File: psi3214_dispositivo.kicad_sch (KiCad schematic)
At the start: 29 parts, among them J1 Screw_Terminal_01x02, J2 Screw_Terminal_01x03, J3 Conn_01x02_Socket, J4 Conn_01x03, J5 Conn_01x02_Socket, J6 Screw_Terminal_01x02, U1 TL072_sim

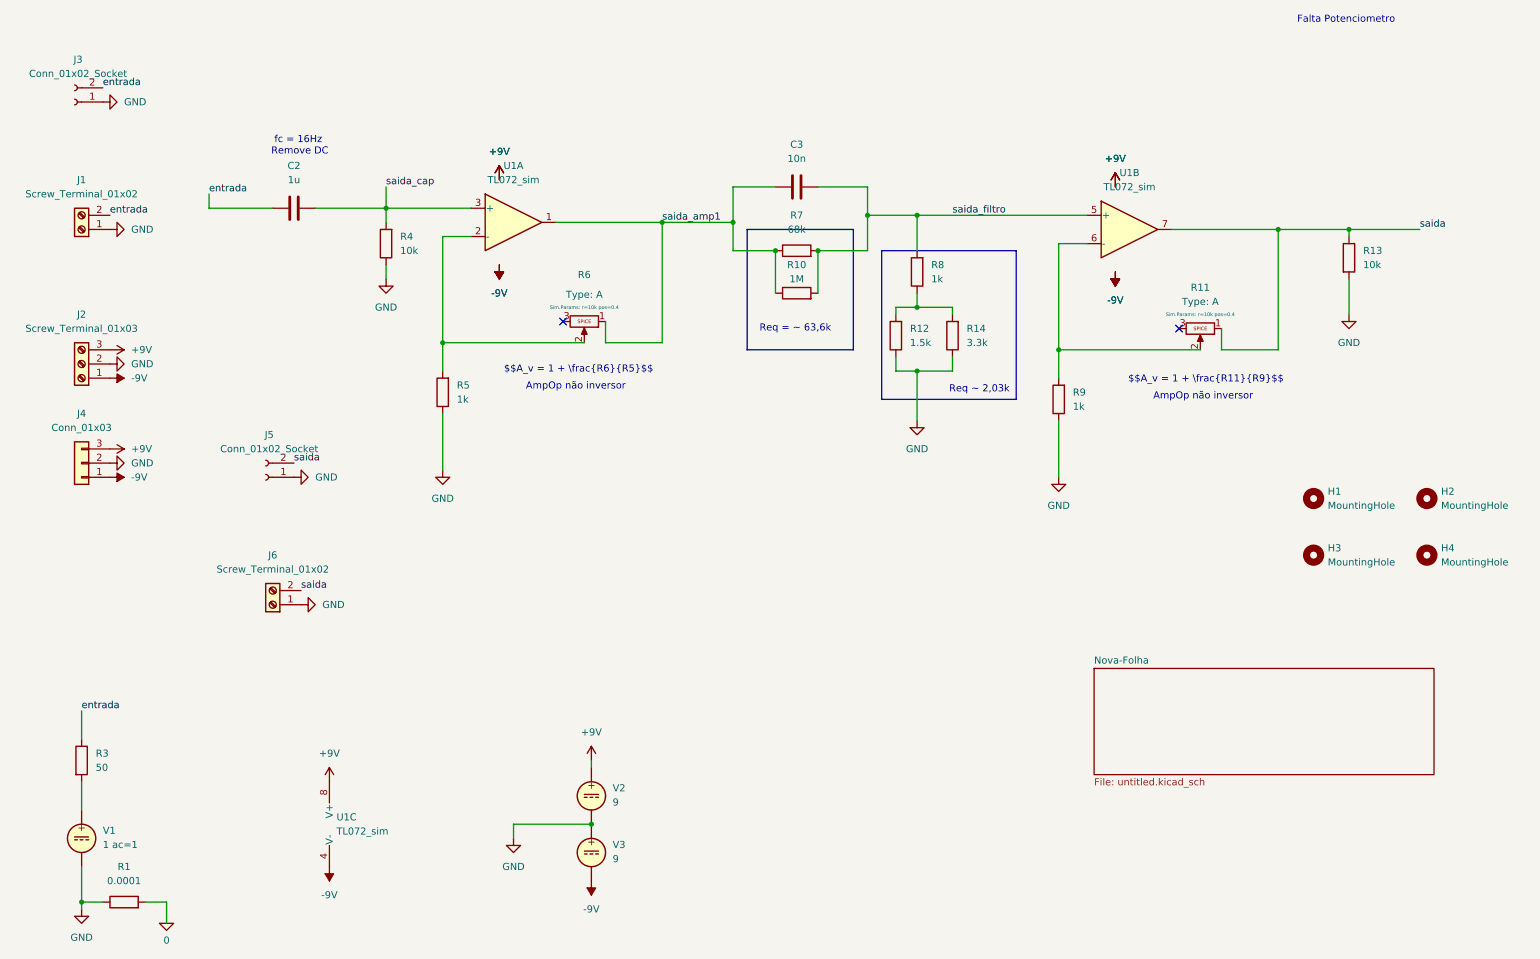
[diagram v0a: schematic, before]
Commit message: Done
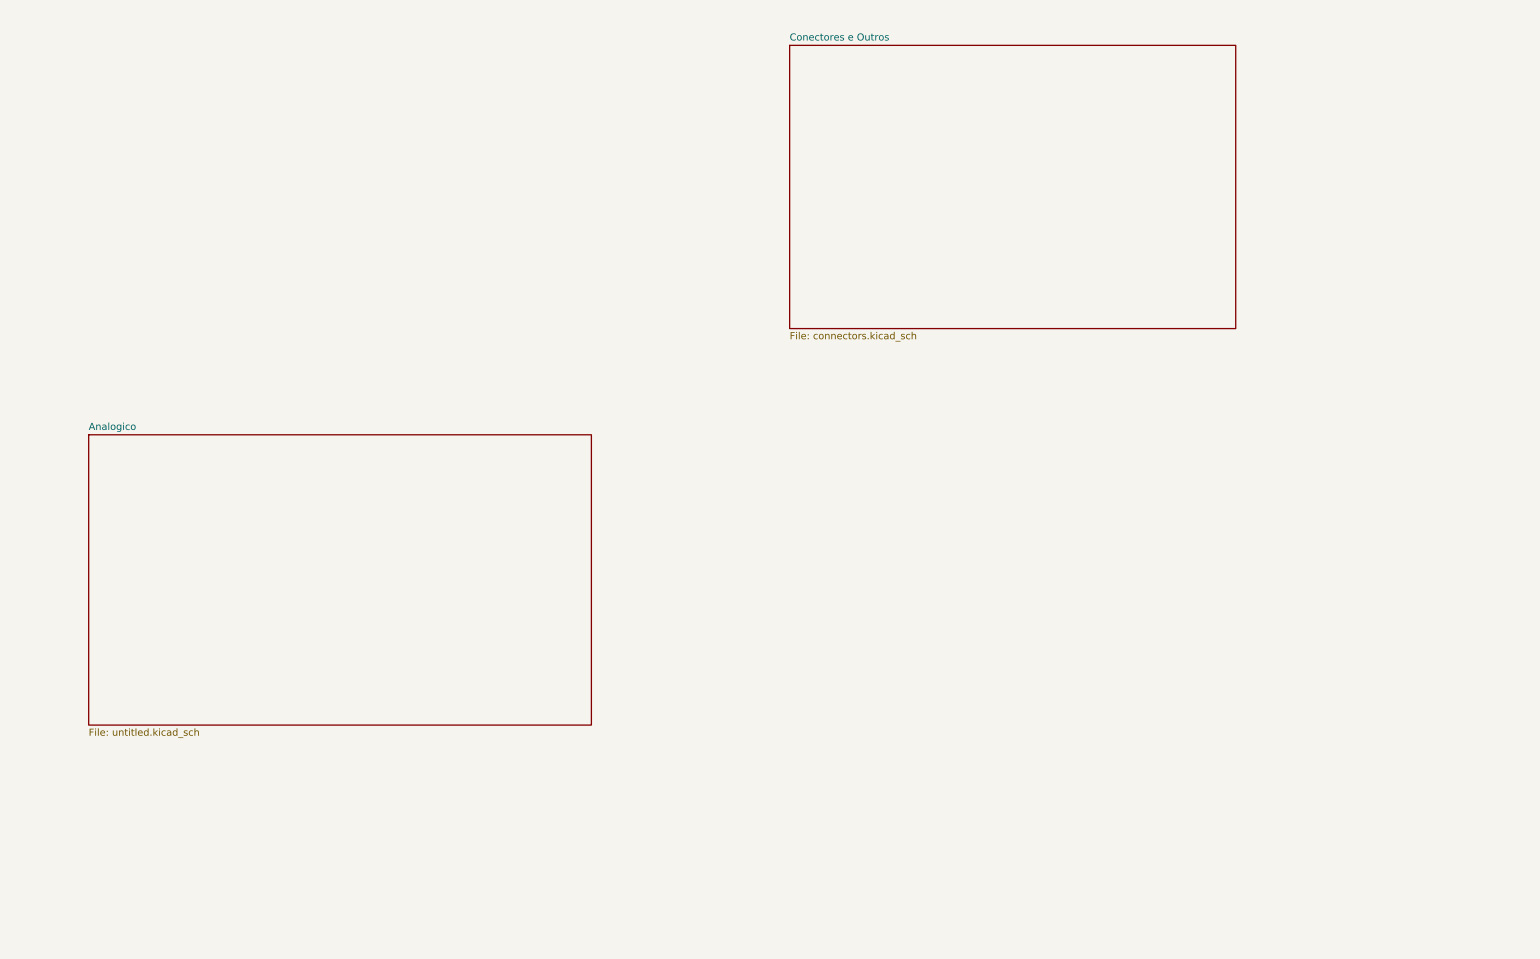
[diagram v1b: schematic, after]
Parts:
- removed C2: 1u, Capacitor_SMD:C_1206_3216Metric, symbol Device:C
- removed C3: 10n, Capacitor_SMD:C_1206_3216Metric, symbol Device:C
- removed H1, H2, H3, H4: MountingHole, MountingHole:MountingHole_3.2mm_M3, symbol Mechanical:MountingHole
- removed J1, J6: Screw_Terminal_01x02, TerminalBlock_Phoenix:TerminalBlock_Phoenix_MKDS-1,5-2-5.08_1x02_P5.08mm_Horizontal, symbol Connector:Screw_Terminal_01x02
- removed J2: Screw_Terminal_01x03, TerminalBlock_Phoenix:TerminalBlock_Phoenix_MKDS-1,5-3-5.08_1x03_P5.08mm_Horizontal, symbol Connector:Screw_Terminal_01x03
- removed J3, J5: Conn_01x02_Socket, Connector_Wire:SolderWire-0.1sqmm_1x02_P3.6mm_D0.4mm_OD1mm, symbol Connector:Conn_01x02_Socket
- removed J4: Conn_01x03, Connector_Wire:SolderWire-0.1sqmm_1x03_P3.6mm_D0.4mm_OD1mm, symbol Connector_Generic:Conn_01x03
- removed R1: 0.0001, symbol Device:R
- removed R10: 1M, Resistor_SMD:R_1206_3216Metric, symbol Device:R
- removed R11, R6: Potentiometer, Potentiometer_THT:Potentiometer_Alps_RK09K_Single_Horizontal, symbol Simulation_SPICE:Potentiometer
- removed R12: 1.5k, Resistor_SMD:R_1206_3216Metric, symbol Device:R
- removed R13, R4: 10k, Resistor_SMD:R_1206_3216Metric, symbol Device:R
- removed R14: 3.3k, Resistor_SMD:R_1206_3216Metric, symbol Device:R
- removed R3: 50, Resistor_SMD:R_1206_3216Metric, symbol Device:R
- removed R5, R8, R9: 1k, Resistor_SMD:R_1206_3216Metric, symbol Device:R
- removed R7: 68k, Resistor_SMD:R_1206_3216Metric, symbol Device:R
- removed U1: TL072_sim, Package_SO:SOIC-8_3.9x4.9mm_P1.27mm, symbol custom:TL072_sim
- removed V1: 1 ac=1, symbol Simulation_SPICE:VDC
- removed V2, V3: 9, symbol Simulation_SPICE:VDC
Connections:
- no-connect marks 2 -> 0
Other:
- removed sheet Nova-Folha
- added sheet Analogico (untitled.kicad_sch)
- added sheet Conectores e Outros (connectors.kicad_sch)
- note removed: "$$A_v = 1 + \frac{R11}{R9}$$"
- note removed: "$$A_v = 1 + \frac{R6}{R5}$$"
- note removed: "AmpOp não inversor"
- note removed: "Falta Potenciometro"
- note removed: "Req = ~ 63,6k"
- note removed: "Req ~ 2,03k"
- note removed: "fc = 16Hz Remove DC"
